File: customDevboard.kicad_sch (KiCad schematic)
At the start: 78 parts, among them J1 USB_C_Receptacle_USB2.0_14P, J10 GPIO29_ADC3, J11 GND, J12 GPIO0, J13 GPIO1, J14 GPIO2, J15 GPIO3, J16 GPIO4, J17 GPIO5, J18 GPIO6, J19 GPIO7, J2 RUN, J20 GPIO8, J21 GPIO9, J22 Conn_01x01, J23 Conn_01x01, J24 Conn_01x01, J25 Conn_01x01, J26 Conn_01x01, J27 Conn_01x01, J28 Conn_01x01, J29 Conn_01x01, J3 3V3, J30 Conn_01x01, J31 Conn_01x01, J32 Conn_01x01, J33 Conn_01x01, J34 Conn_01x01, J35 Conn_01x01, J36 Conn_01x01, J37 Conn_01x01, J38 Conn_01x01, J39 Conn_01x01, J4 VBUS, J40 Conn_01x01, J41 Conn_01x01, J42 SWCLK, J43 GND, J44 SWD, J5 GND, J6 GND, J7 GPIO26_ADC0, J8 GPIO27_ADC1, J9 GPIO28_ADC2, SW1 BOOT, U1 RP2040, U2 W25Q128JVP, U3 TLV75733PDRV, Y1 12 MHz

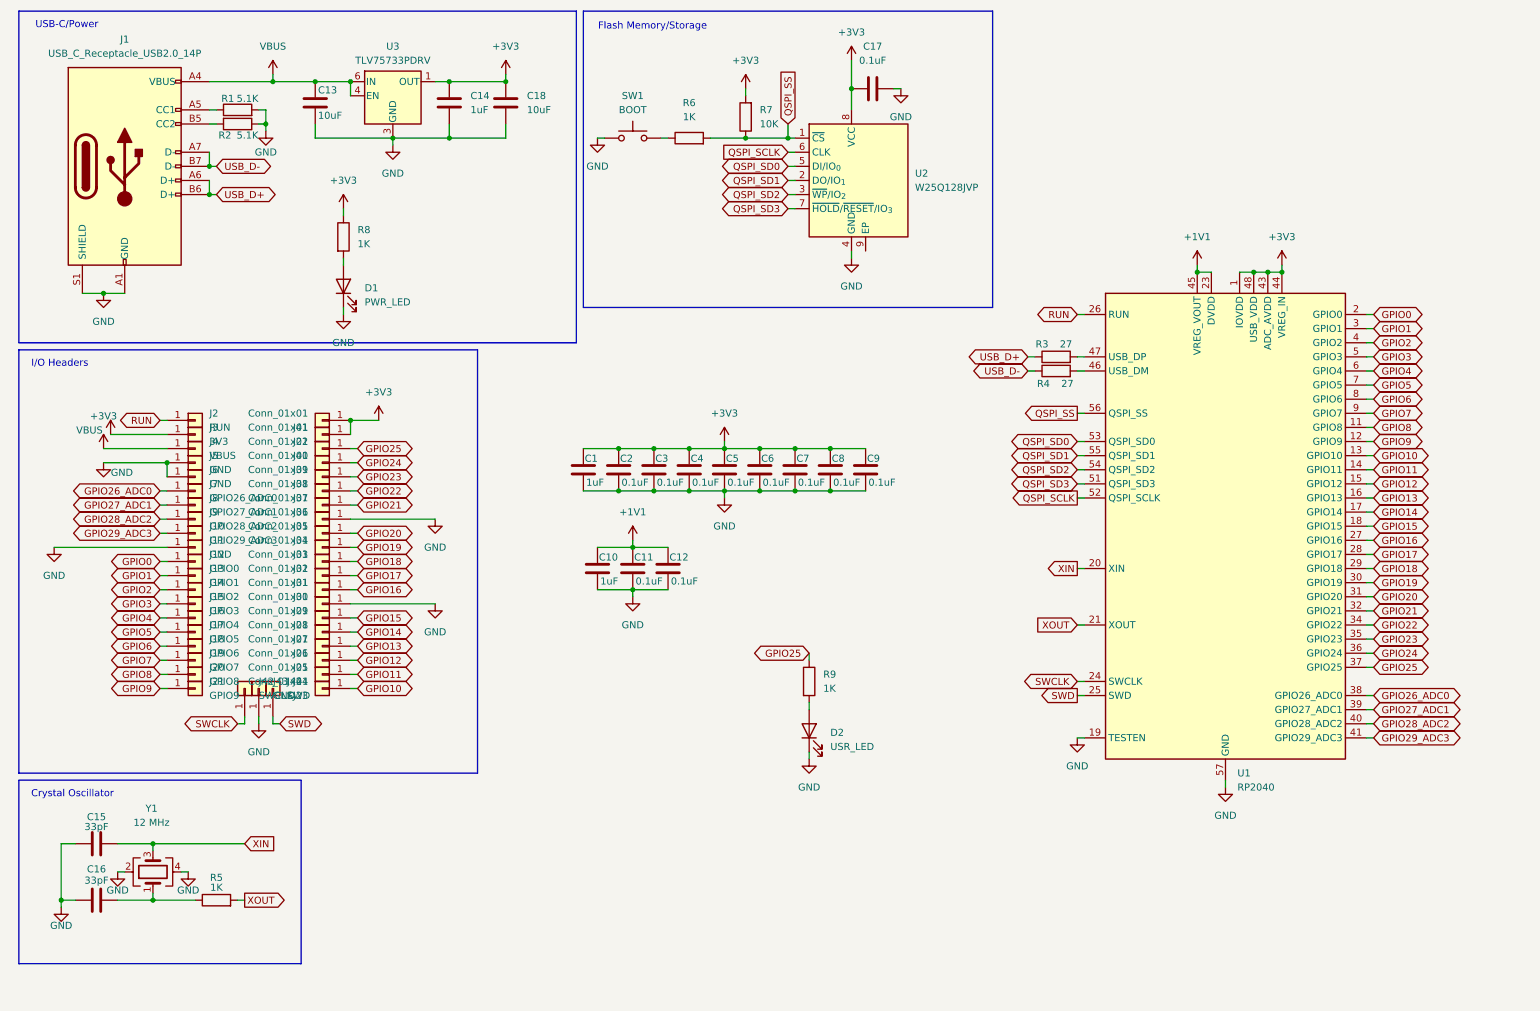
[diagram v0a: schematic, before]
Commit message: optimise
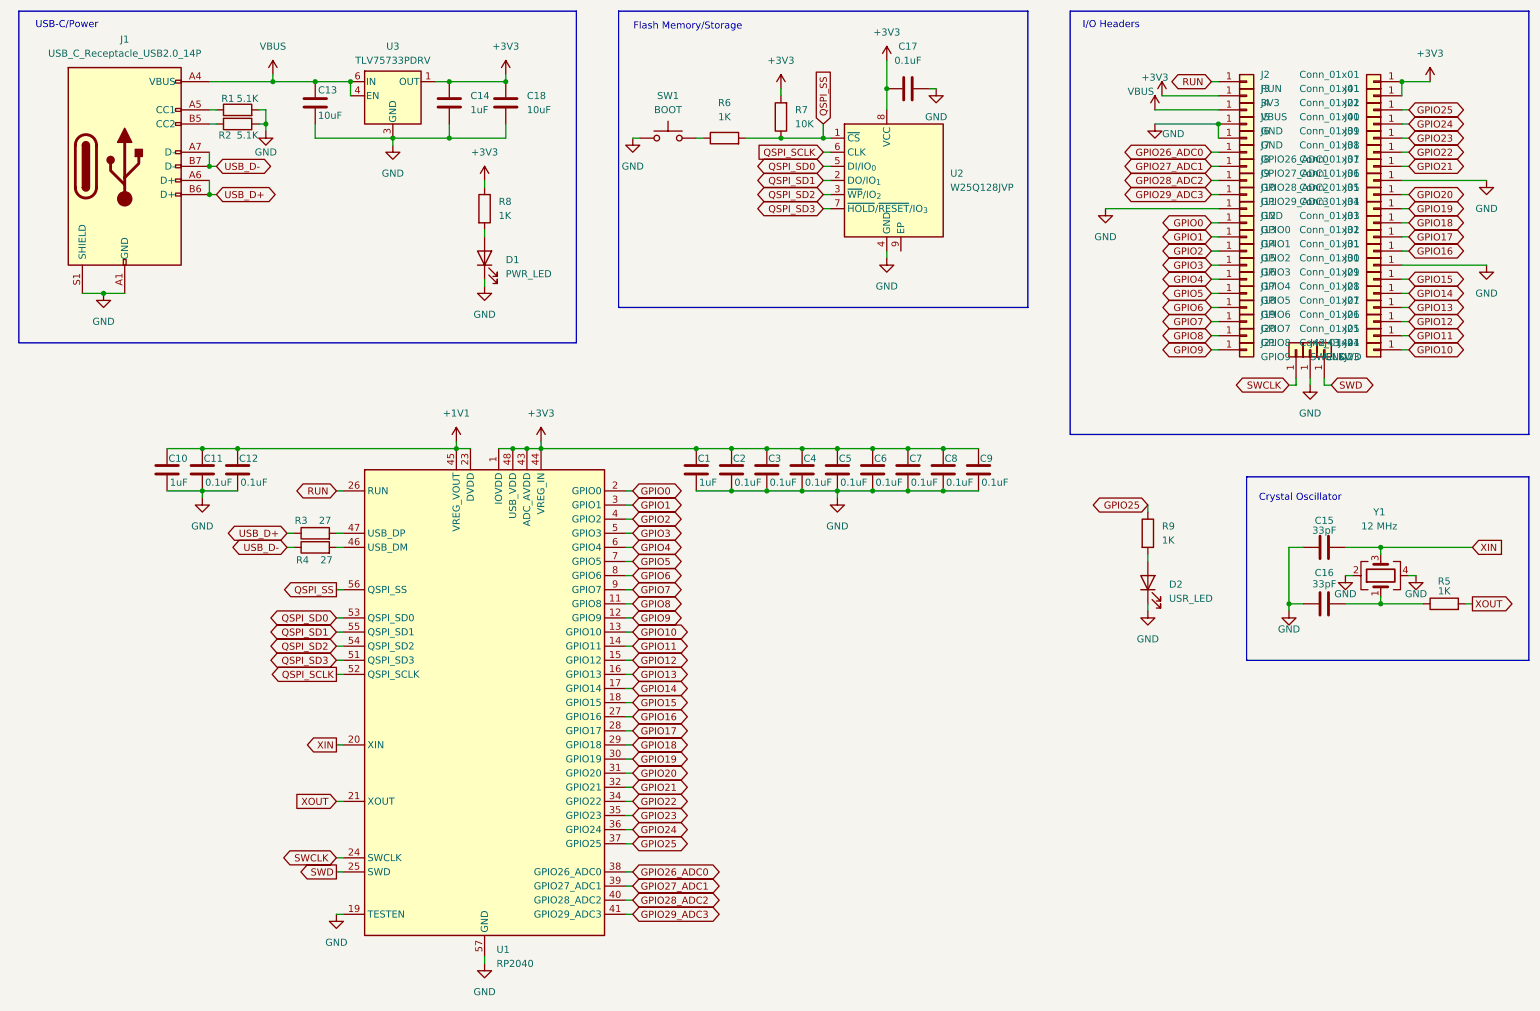
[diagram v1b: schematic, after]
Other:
- moved on the sheet: C1, C10, C11, C12, C15, C16, C17, C2, C3, C4, C5, C6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
